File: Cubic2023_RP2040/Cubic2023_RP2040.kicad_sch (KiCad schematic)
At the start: 33 parts, among them J1 Conn_02x06_Odd_Even, J2 Conn_02x06_Odd_Even, J3 MICROXNJ, J4 Conn_02x06_Odd_Even, SW1 SW_Push, SW2 SW_Push, U1 RP2040, U3 W25Q128JVS, Y1 12MHz_Crystal

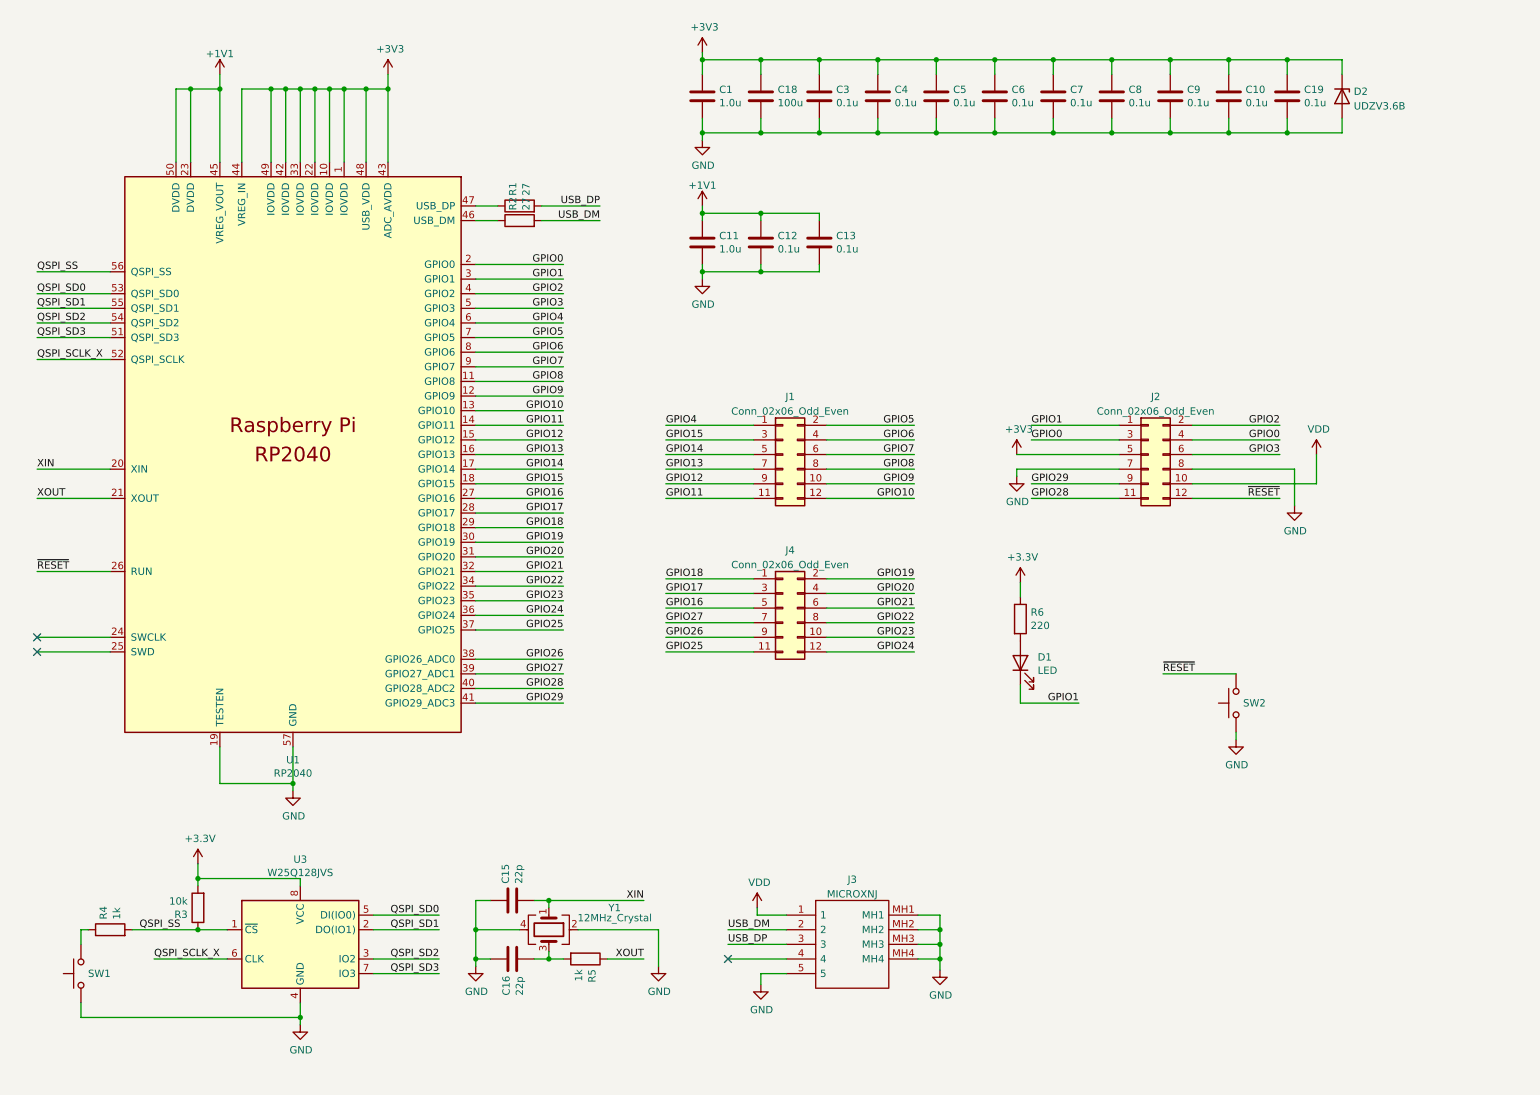
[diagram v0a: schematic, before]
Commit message: WIP
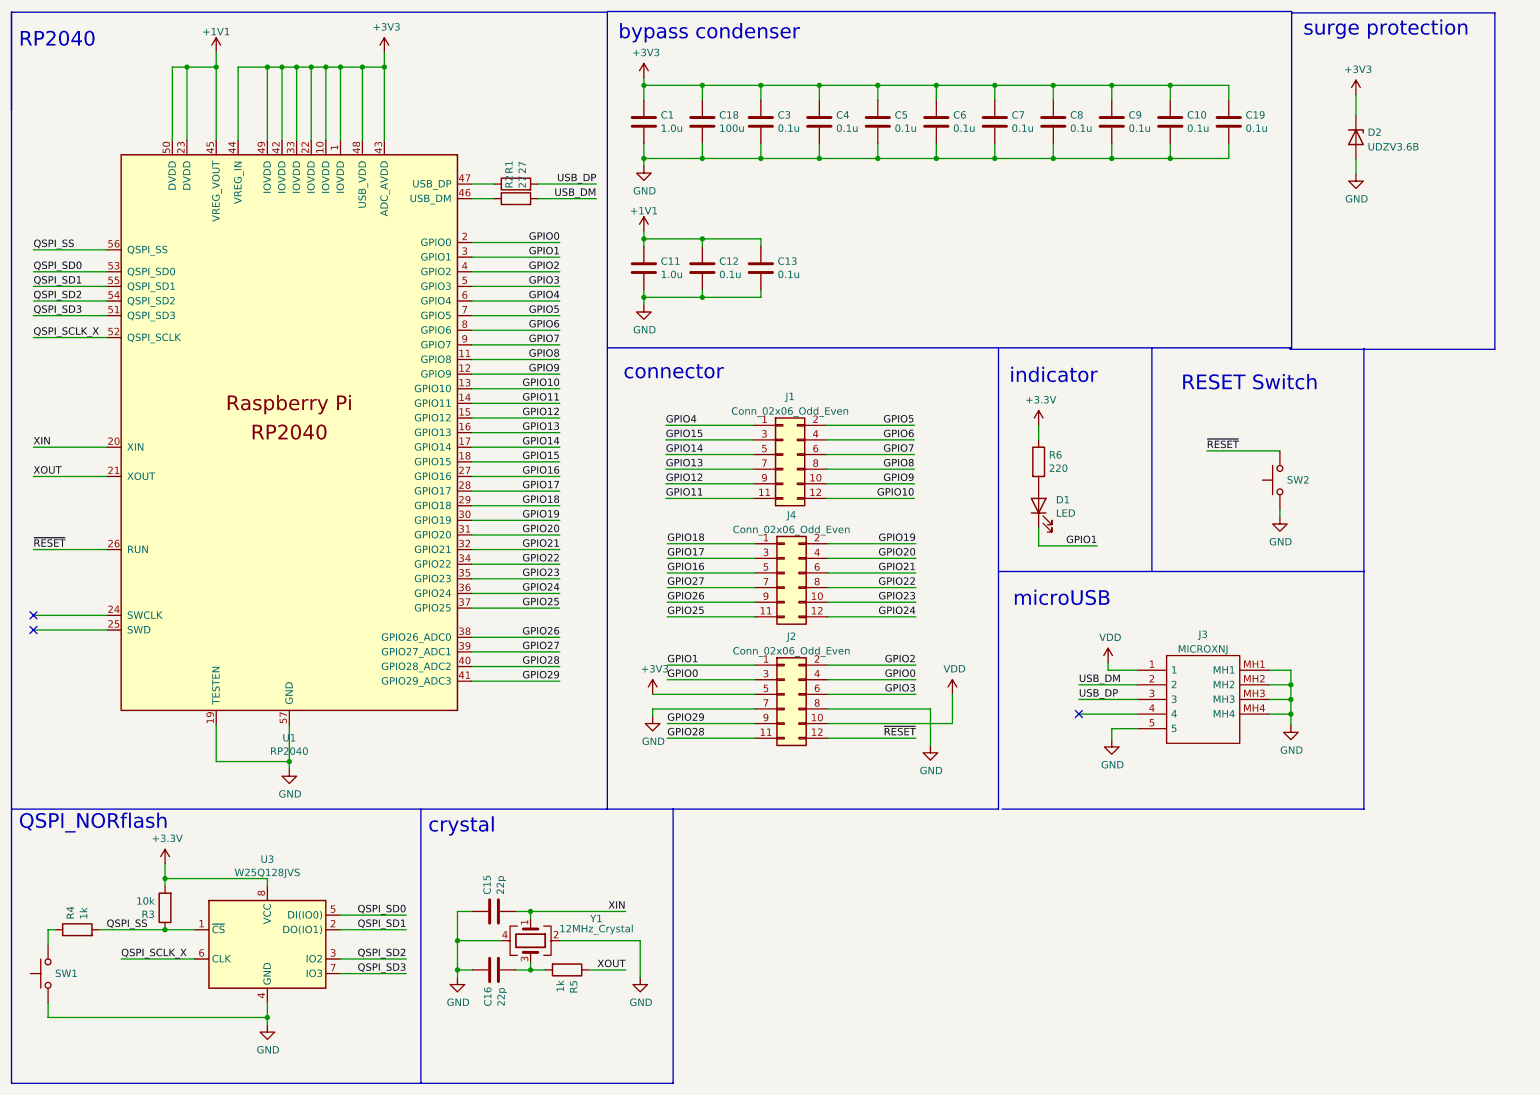
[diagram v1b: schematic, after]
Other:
- note added: "QSPI_NORflash"
- note added: "RESET Switch"
- note added: "RP2040"
- note added: "bypass condenser"
- note added: "connector"
- note added: "crystal"
- note added: "indicator"
- note added: "microUSB"
- note added: "surge protection"
- moved on the sheet: C1, C10, C11, C12, C13, C15, C16, C18, C19, C3, C4, C5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
